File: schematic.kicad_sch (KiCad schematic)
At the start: 60 parts, among them J2 Audio Out, J4 Audio In, Q2 2N5457 (JFET), Q3 2N5457 (JFET), Q4 2N5457 (JFET), Q5 2N5457 (JFET), Q6 2N3904, Q7 2N3904, Q8 2N3904, SW1 SW_SPST, U1 LM741, U2 LM741, U3 LM741, U4 LM741, U5 LM741

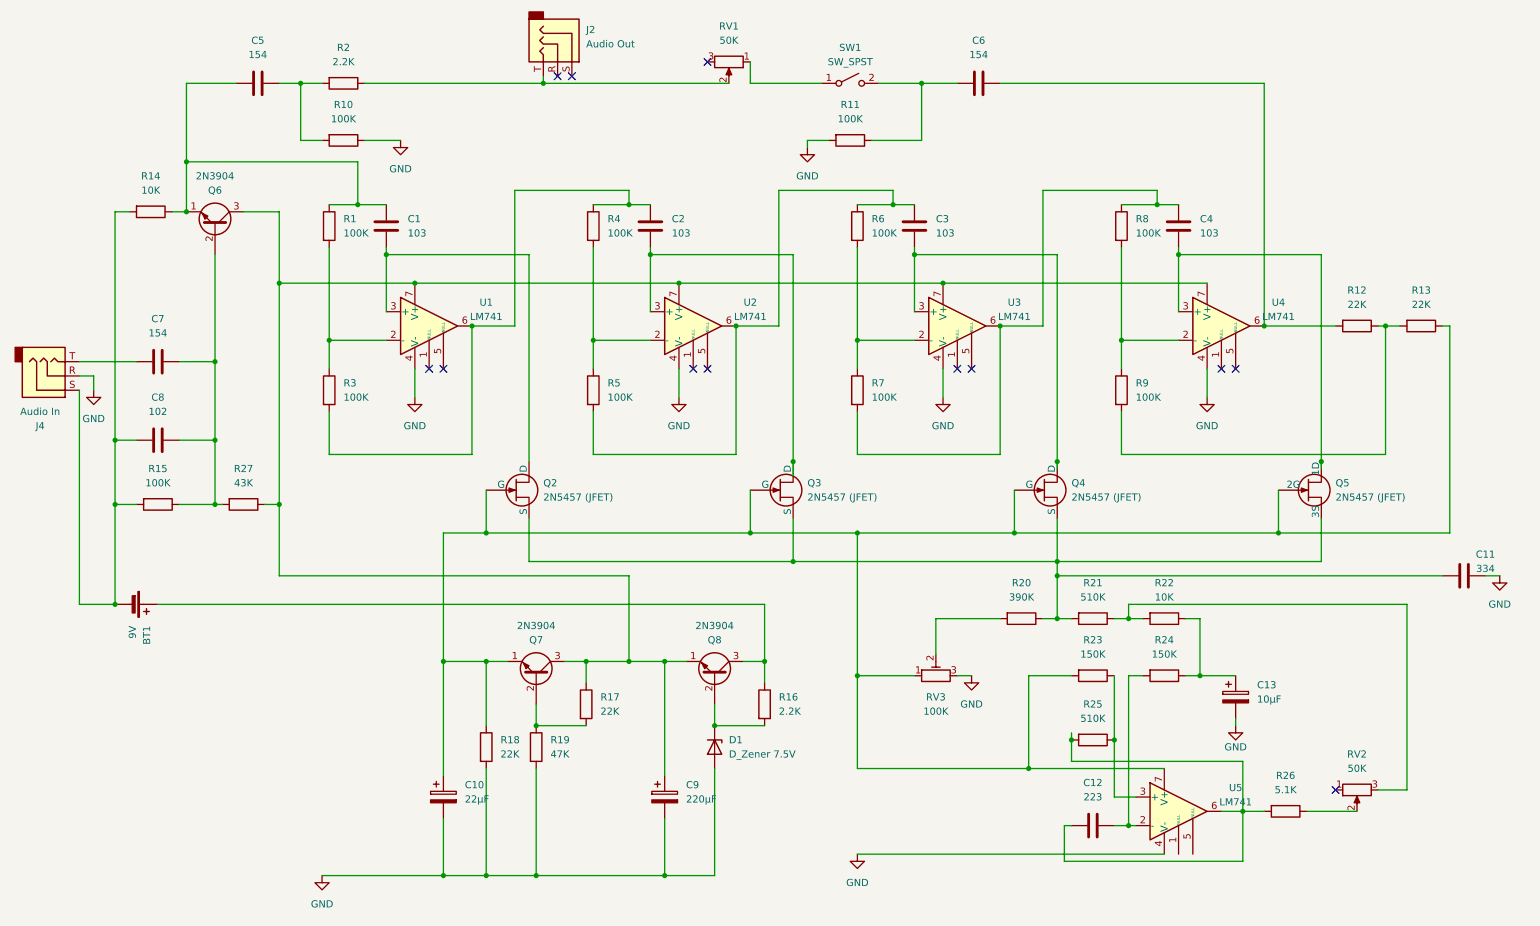
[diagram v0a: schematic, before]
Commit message: update
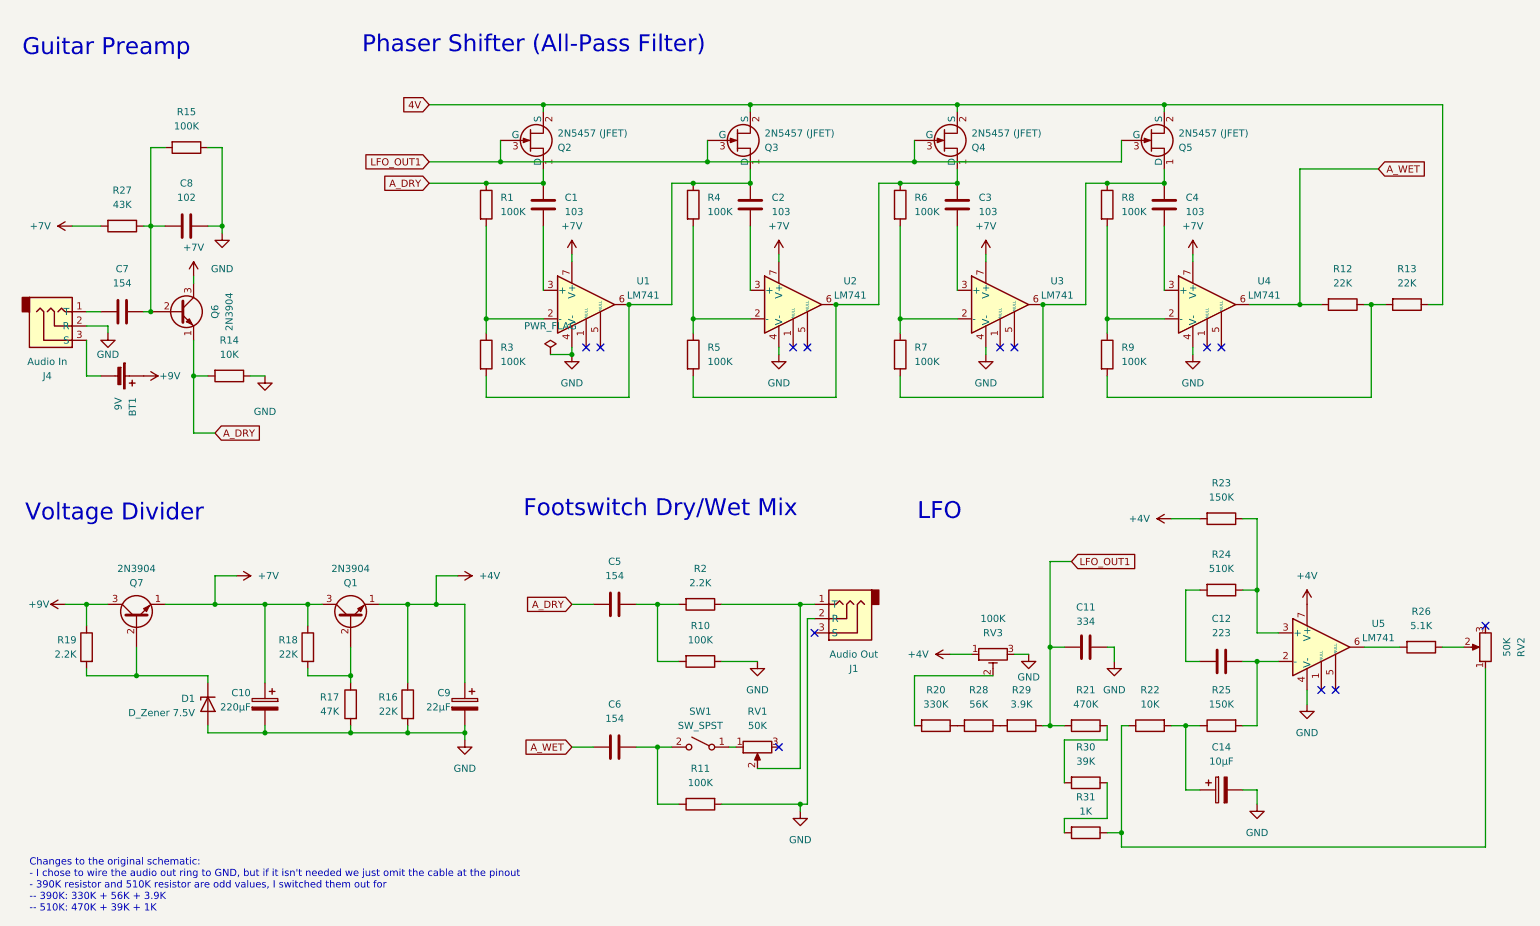
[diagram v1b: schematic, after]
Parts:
- removed C13: 10µF, Capacitor_THT:CP_Radial_D5.0mm_P2.50mm, symbol Device:C_Polarized
- removed J2: Audio Out, Library:AudioMountPoint2, symbol Connector_Audio:AudioJack3
- removed Q8: 2N3904, Package_TO_SOT_THT:TO-92_Inline_Wide, symbol Transistor_BJT:2N3904
- added C14: 10µF, Capacitor_THT:CP_Radial_D5.0mm_P2.50mm, symbol Device:C_Polarized
- added J1: Audio Out, Connector_PinHeader_2.54mm:PinHeader_1x02_P2.54mm_Vertical, symbol Connector_Audio:AudioJack3
- added Q1: 2N3904, Package_TO_SOT_THT:TO-92_Inline, symbol Transistor_BJT:2N3904
- added R28: 56K, Resistor_THT:R_Axial_DIN0204_L3.6mm_D1.6mm_P5.08mm_Horizontal, symbol Device:R
- added R29: 3.9K, Resistor_THT:R_Axial_DIN0204_L3.6mm_D1.6mm_P5.08mm_Horizontal, symbol Device:R
- added R30: 39K, Resistor_THT:R_Axial_DIN0204_L3.6mm_D1.6mm_P5.08mm_Horizontal, symbol Device:R
- added R31: 1K, Resistor_THT:R_Axial_DIN0204_L3.6mm_D1.6mm_P5.08mm_Horizontal, symbol Device:R
- BT1, SW1: footprint LED_THT:LED_D2.0mm_W4.8mm_H2.5mm_FlatTop -> Connector_PinHeader_2.54mm:PinHeader_1x02_P2.54mm_Vertical
- C1, C2, C3, C4: footprint Resistor_THT:R_Axial_DIN0207_L6.3mm_D2.5mm_P7.62mm_Horizontal -> Capacitor_THT:C_Axial_L5.1mm_D3.1mm_P7.50mm_Horizontal
- C10: value 22µF -> 220µF; footprint Capacitor_THT:CP_Radial_D5.0mm_P2.50mm -> Capacitor_THT:CP_Radial_D10.0mm_P5.00mm
- C11, C5, C6, C7: footprint Resistor_THT:R_Axial_DIN0207_L6.3mm_D2.5mm_P5.08mm_Vertical -> Capacitor_THT:C_Disc_D3.0mm_W1.6mm_P2.50mm
- C12, C8: footprint Resistor_THT:R_Axial_DIN0207_L6.3mm_D2.5mm_P5.08mm_Vertical -> Capacitor_THT:C_Axial_L5.1mm_D3.1mm_P7.50mm_Horizontal
- C9: value 220µF -> 22µF; footprint Capacitor_THT:CP_Radial_D10.0mm_P5.00mm -> Capacitor_THT:CP_Radial_D5.0mm_P2.50mm
- D1: footprint Resistor_THT:R_Axial_DIN0207_L6.3mm_D2.5mm_P5.08mm_Vertical -> Diode_THT:D_A-405_P7.62mm_Horizontal
- J4: footprint Library:AudioMountPoint2 -> Connector_PinHeader_2.54mm:PinHeader_1x03_P2.54mm_Vertical
- Q2, Q3, Q4, Q5, Q6, Q7: footprint Package_TO_SOT_THT:TO-92_Inline_Wide -> Package_TO_SOT_THT:TO-92_Inline
- R1, R10, R11, R12, R14, R2, R22, R23, R26, R3, R4, R5, R6, R7, R8, R9: footprint Resistor_THT:R_Axial_DIN0207_L6.3mm_D2.5mm_P7.62mm_Horizontal -> Resistor_THT:R_Axial_DIN0204_L3.6mm_D1.6mm_P5.08mm_Horizontal
- R13, R15: footprint Resistor_THT:R_Axial_DIN0207_L6.3mm_D2.5mm_P5.08mm_Vertical -> Resistor_THT:R_Axial_DIN0204_L3.6mm_D1.6mm_P5.08mm_Horizontal
- R16: value 2.2K -> 22K; footprint Resistor_THT:R_Axial_DIN0207_L6.3mm_D2.5mm_P2.54mm_Vertical -> Resistor_THT:R_Axial_DIN0204_L3.6mm_D1.6mm_P5.08mm_Horizontal
- R17: value 22K -> 47K; footprint Resistor_THT:R_Axial_DIN0207_L6.3mm_D2.5mm_P2.54mm_Vertical -> Resistor_THT:R_Axial_DIN0204_L3.6mm_D1.6mm_P5.08mm_Horizontal
- R18, R27: footprint Resistor_THT:R_Axial_DIN0207_L6.3mm_D2.5mm_P2.54mm_Vertical -> Resistor_THT:R_Axial_DIN0204_L3.6mm_D1.6mm_P5.08mm_Horizontal
- R19: value 47K -> 2.2K; footprint Resistor_THT:R_Axial_DIN0207_L6.3mm_D2.5mm_P2.54mm_Vertical -> Resistor_THT:R_Axial_DIN0204_L3.6mm_D1.6mm_P5.08mm_Horizontal
- R20: value 390K -> 330K; footprint Resistor_THT:R_Axial_DIN0207_L6.3mm_D2.5mm_P7.62mm_Horizontal -> Resistor_THT:R_Axial_DIN0204_L3.6mm_D1.6mm_P5.08mm_Horizontal
- R21: value 510K -> 470K; footprint Resistor_THT:R_Axial_DIN0207_L6.3mm_D2.5mm_P7.62mm_Horizontal -> Resistor_THT:R_Axial_DIN0204_L3.6mm_D1.6mm_P5.08mm_Horizontal
- R24: value 150K -> 510K; footprint Resistor_THT:R_Axial_DIN0207_L6.3mm_D2.5mm_P2.54mm_Vertical -> Resistor_THT:R_Axial_DIN0204_L3.6mm_D1.6mm_P5.08mm_Horizontal
- R25: value 510K -> 150K; footprint Resistor_THT:R_Axial_DIN0207_L6.3mm_D2.5mm_P2.54mm_Vertical -> Resistor_THT:R_Axial_DIN0204_L3.6mm_D1.6mm_P5.08mm_Horizontal
- RV1, RV2: footprint Potentiometer_THT:Potentiometer_Bourns_3266Y_Vertical -> Connector_PinHeader_2.54mm:PinHeader_1x02_P2.54mm_Vertical
- RV3: footprint Potentiometer_THT:Potentiometer_Runtron_RM-065_Vertical -> Potentiometer_THT:Potentiometer_Runtron_RM-063_Horizontal
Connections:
- net GND: now also C8.1, J4.2 (R), R14.1, R15.1, R16.2, R17.2, C14.2, J1.2 (R); no longer J4.R, R18.2, R19.2
- net at C3.1, R5.2, R6.1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: now also Q4.1 (D)
- net A_DRY: now reaches C1.1, C5.2, Q6.1 (E), R1.1
- net A_DRY: now also Q2.1 (D), R14.2; no longer R14.1
- net +7V: now reaches Q6.3 (C), U1.7 (V+), U2.7 (V+), U3.7 (V+), U4.7 (V+)
- net +7V: now also C10.1, Q7.1 (E), R18.1, R27.2, Q1.3 (C); no longer C9.1, Q7.3 (C), R17.1, R27.1
- net at D1.1 (K): now also Q7.2 (B), R19.2; no longer R16.2
- net +4V: now reaches R16.1
- net +4V: now also C9.1, R23.2, RV3.1, U5.7 (V+), Q1.1 (E); no longer BT1.1 (+)
- net at C2.2, U2.3 (+): no longer Q3.1 (D)
- net at R2.1, RV1.2: now also J1.1 (T)
- net at C1.2, U1.3 (+): no longer Q2.1 (D)
- net LFO_OUT1: now reaches C11.2, Q2.3 (G), Q3.3 (G), Q4.3 (G), Q5.3 (G), R21.2
- net LFO_OUT1: now also R29.1; no longer R20.1
- net at C2.1, R3.2, R4.1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: now also Q3.1 (D)
- net A_WET: now reaches C6.1, R12.2, U4.6
- net at C4.1, R7.2, R8.1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: now also Q5.1 (D)
- net at C4.2, U4.3 (+): no longer Q5.1 (1D)
- net at C3.2, U3.3 (+): no longer Q4.1 (D)
- net at R22.1: now also RV2.1, R31.1; no longer R24.1
- net at C12.1, U5.2 (-): now also R25.2; no longer R24.2
- net at R23.1, U5.3 (+): now also R24.1; no longer R25.1
- net at R26.2, U5.6: no longer C12.2, R25.2
- net at C7.2: now also J4.1 (T); no longer J4.T
- new net: C7.1, C8.2, Q6.2 (B), R15.2, R27.1
- new net: Q1.2 (B), R17.1, R18.2
- new net: R30.1, R31.2
- new net: R20.1, R28.2
- new net: C12.2, R24.2
- new net: R28.1, R29.2
- new net: R21.1, R30.2
- new net: C14.1, R22.2, R25.1
- new net: BT1.2 (-), J4.3 (S)
- new net +9V: BT1.1 (+), Q7.3 (C), R19.1
- new net 4V: Q2.2 (S), Q3.2 (S), Q4.2 (S), Q5.2 (S), R13.1
- now unconnected: RV2.3
- no-connect marks 12 -> 13
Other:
- note added: "Changes to the original schematic: - I chose to wire the audio out ring to GND, but if it isn't needed we just omit the cable at the pinout - 390K resistor and 510K resistor are odd values, I switched them out for -- 390K: 330K + 56K + 3.9K -- 510K: 470K + 39K + 1K"
- note added: "Footswitch Dry/Wet Mix"
- note added: "Guitar Preamp"
- note added: "LFO"
- note added: "Phaser Shifter (All-Pass Filter)"
- note added: "Voltage Divider"
- moved on the sheet: BT1, C1, C2, C3, C4, C5, C6, C8, R1, R10, R11, R12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
